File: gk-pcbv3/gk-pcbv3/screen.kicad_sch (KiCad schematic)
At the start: 10 parts, among them J3 Conn_02x15_Counter_Clockwise, U11 ULN2003A

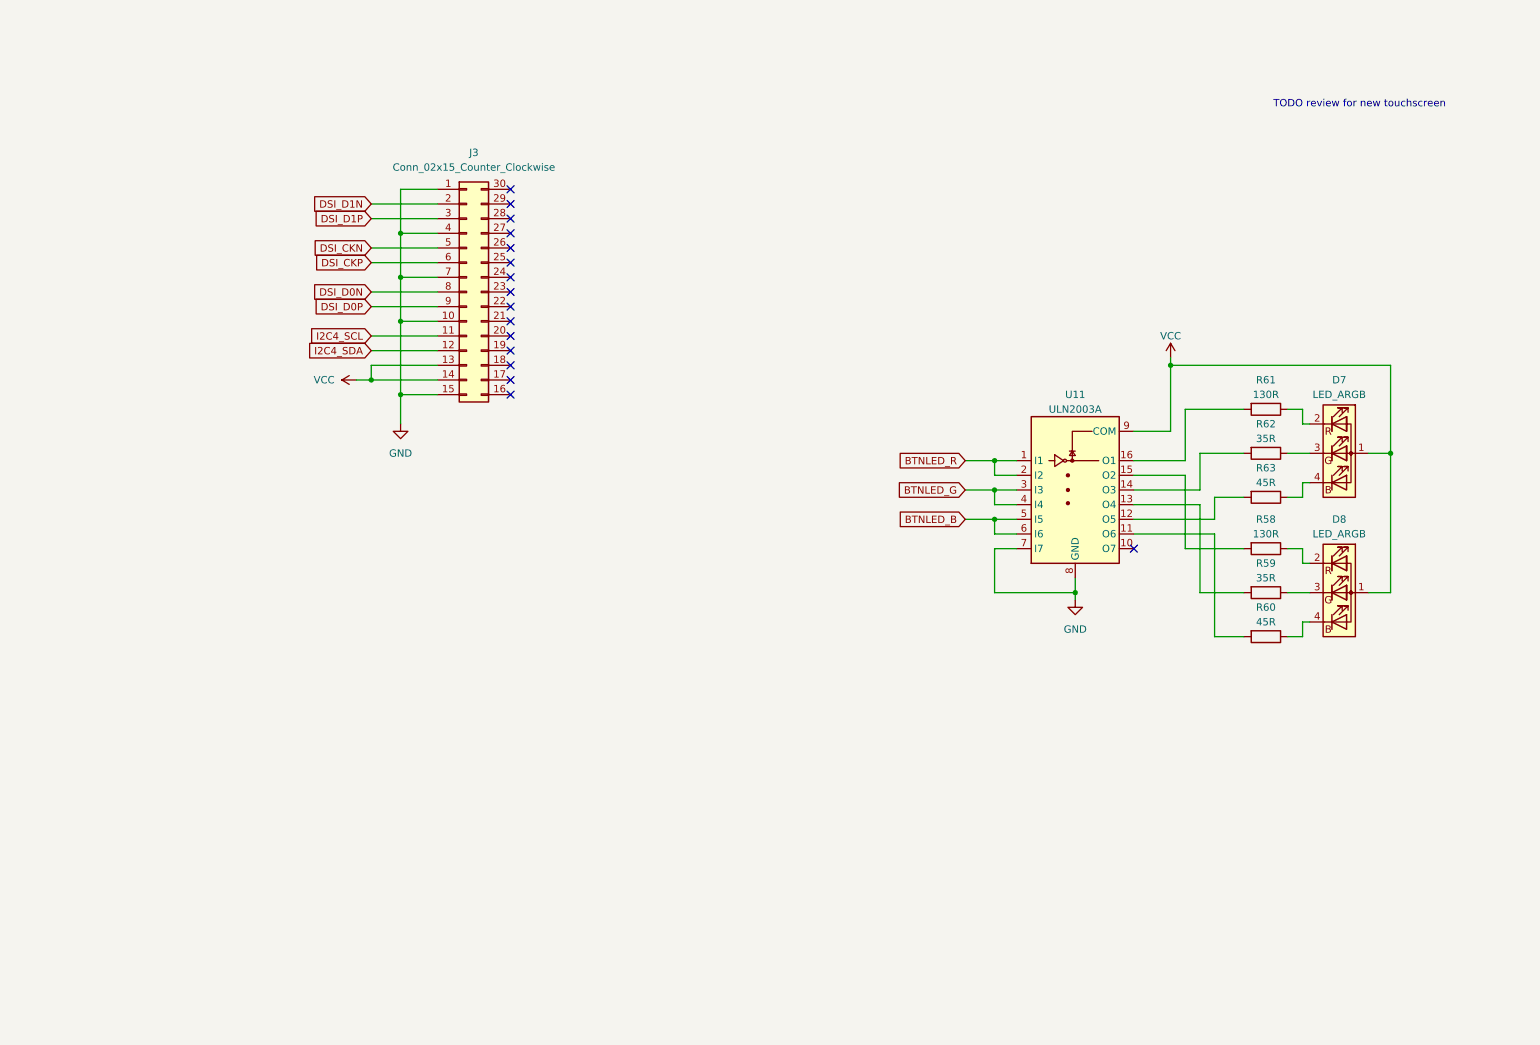
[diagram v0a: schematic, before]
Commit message: v3 board
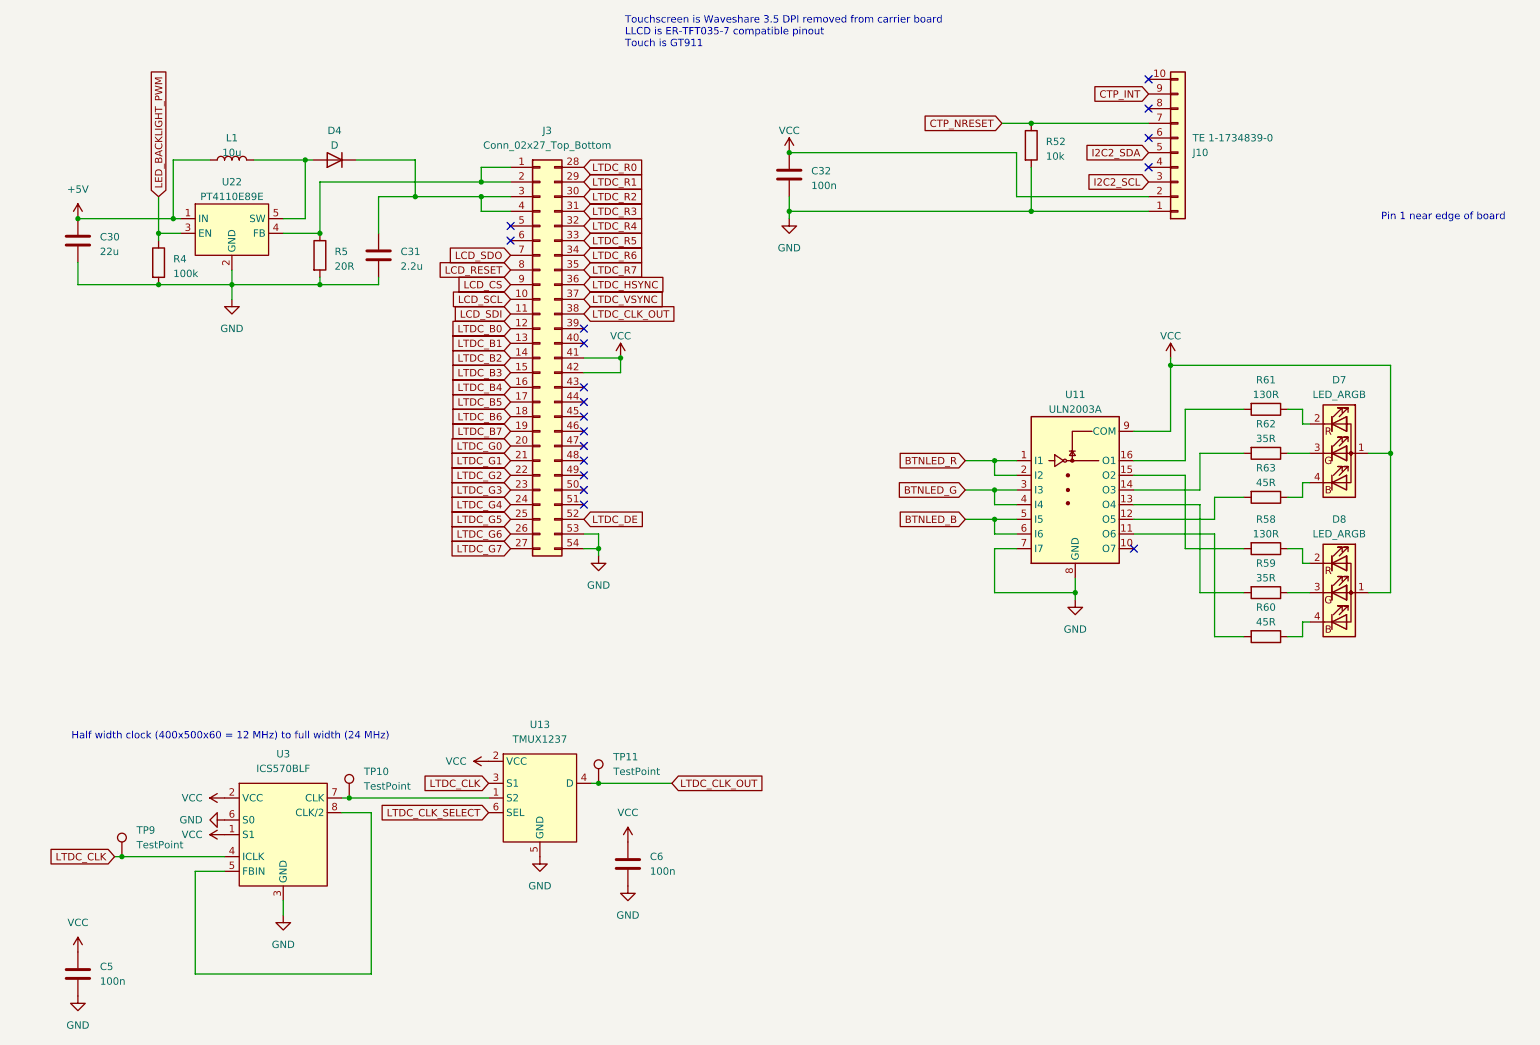
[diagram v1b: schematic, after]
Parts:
- removed J3: Conn_02x15_Counter_Clockwise, symbol Connector_Generic:Conn_02x15_Counter_Clockwise
- added C30: 22u, Capacitor_SMD:C_0805_2012Metric, symbol Device:C
- added C31: 2.2u, Capacitor_SMD:C_0805_2012Metric, symbol Device:C
- added C32, C5, C6: 100n, Capacitor_SMD:C_0603_1608Metric, symbol Device:C
- added D4: D, Diode_SMD:D_SOD-128, symbol Device:D
- added J10: TE 1-1734839-0, Connector_FFC-FPC:TE_1-1734839-0_1x10-1MP_P0.5mm_Horizontal, symbol Connector_Generic:Conn_01x10
- added J3: Conn_02x27_Top_Bottom, amphenol:AMPHENOL_F32Q-1A7H1-11054, symbol Connector_Generic:Conn_02x27_Top_Bottom
- added L1: 10u, Inductor_SMD:L_7.3x7.3_H3.5, symbol Device:L
- added R4: 100k, Resistor_SMD:R_0603_1608Metric, symbol Device:R
- added R5: 20R, Resistor_SMD:R_2512_6332Metric, symbol Device:R
- added R52: 10k, Resistor_SMD:R_0603_1608Metric, symbol Device:R
- added TP10, TP11, TP9: TestPoint, TestPoint:TestPoint_Pad_D1.0mm, symbol Connector:TestPoint
- added U13: TMUX1237, Package_TO_SOT_SMD:SOT-363_SC-70-6, symbol gk-syms:TMUX1237
- added U22: PT4110E89E, Package_TO_SOT_SMD:SOT-89-5, symbol gk-syms:PT4110
- added U3: ICS570BLF, Package_SO:SO-8_3.9x4.9mm_P1.27mm, symbol gk-syms:ICS570BLF
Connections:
- net GND: now also C30.2, C31.2, C32.2, C5.2, C6.2, J10.1 (Pin_1), J3.53 (Pin_53), J3.54 (Pin_54), R4.2, R5.2, R52.2, U13.5 (GND), U22.2 (GND), U3.3 (GND), U3.6 (S0)
- net VCC: now also C32.1, C5.1, C6.1, J10.2 (Pin_2), J3.41 (Pin_41), J3.42 (Pin_42), U13.2 (VCC), U3.1 (S1), U3.2 (VCC)
- new net: J3.1 (Pin_1), J3.2 (Pin_2), R5.1, U22.4 (FB)
- new net: D4.2 (A), L1.2, U22.5 (SW)
- new net: TP10.1, U13.1 (S2), U3.7 (CLK)
- new net: U3.5 (FBIN), U3.8 (CLK/2)
- new net: C31.1, D4.1 (K), J3.3 (Pin_3), J3.4 (Pin_4)
- new net +5V: C30.1, L1.1, U22.1 (IN)
- new net CTP_INT: J10.9 (Pin_9)
- new net CTP_NRESET: J10.7 (Pin_7), R52.1
- new net I2C2_SCL: J10.3 (Pin_3)
- new net I2C2_SDA: J10.5 (Pin_5)
- new net LCD_CS: J3.9 (Pin_9)
- new net LCD_RESET: J3.8 (Pin_8)
- new net LCD_SCL: J3.10 (Pin_10)
- new net LCD_SDI: J3.11 (Pin_11)
- new net LCD_SDO: J3.7 (Pin_7)
- new net LED_BACKLIGHT_PWM: R4.1, U22.3 (EN)
- new net LTDC_B0: J3.12 (Pin_12)
- new net LTDC_B1: J3.13 (Pin_13)
- new net LTDC_B2: J3.14 (Pin_14)
- new net LTDC_B3: J3.15 (Pin_15)
- new net LTDC_B4: J3.16 (Pin_16)
- new net LTDC_B5: J3.17 (Pin_17)
- new net LTDC_B6: J3.18 (Pin_18)
- new net LTDC_B7: J3.19 (Pin_19)
- new net LTDC_CLK: TP9.1, U13.3 (S1), U3.4 (ICLK)
- new net LTDC_CLK_OUT: J3.38 (Pin_38), TP11.1, U13.4 (D)
- new net LTDC_CLK_SELECT: U13.6 (SEL)
- new net LTDC_DE: J3.52 (Pin_52)
- new net LTDC_G0: J3.20 (Pin_20)
- new net LTDC_G1: J3.21 (Pin_21)
- new net LTDC_G2: J3.22 (Pin_22)
- new net LTDC_G3: J3.23 (Pin_23)
- new net LTDC_G4: J3.24 (Pin_24)
- new net LTDC_G5: J3.25 (Pin_25)
- new net LTDC_G6: J3.26 (Pin_26)
- new net LTDC_G7: J3.27 (Pin_27)
- new net LTDC_HSYNC: J3.36 (Pin_36)
- new net LTDC_R0: J3.28 (Pin_28)
- new net LTDC_R1: J3.29 (Pin_29)
- new net LTDC_R2: J3.30 (Pin_30)
- new net LTDC_R3: J3.31 (Pin_31)
- new net LTDC_R4: J3.32 (Pin_32)
- new net LTDC_R5: J3.33 (Pin_33)
- new net LTDC_R6: J3.34 (Pin_34)
- new net LTDC_R7: J3.35 (Pin_35)
- new net LTDC_VSYNC: J3.37 (Pin_37)
- no-connect marks 16 -> 18
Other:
- note added: "Half width clock (400x500x60 = 12 MHz) to full width (24 MHz)"
- note added: "Pin 1 near edge of board"
- note added: "Touchscreen is Waveshare 3.5 DPI removed from carrier board LLCD is ER-TFT035-7 compatible pinout Touch is GT911"
- note removed: "TODO review for new touchscreen"
